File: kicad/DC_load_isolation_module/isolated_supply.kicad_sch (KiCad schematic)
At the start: 53 parts, among them Q10 AO3400A, Q11 AO3400A, Q12 MMBT5551L, Q14 MMBT5401, Q15 MMBT5551L, Q16 MMBT5551L, Q8 MMBT5551L, Q9 MMBT5401, U5 74HC14D653

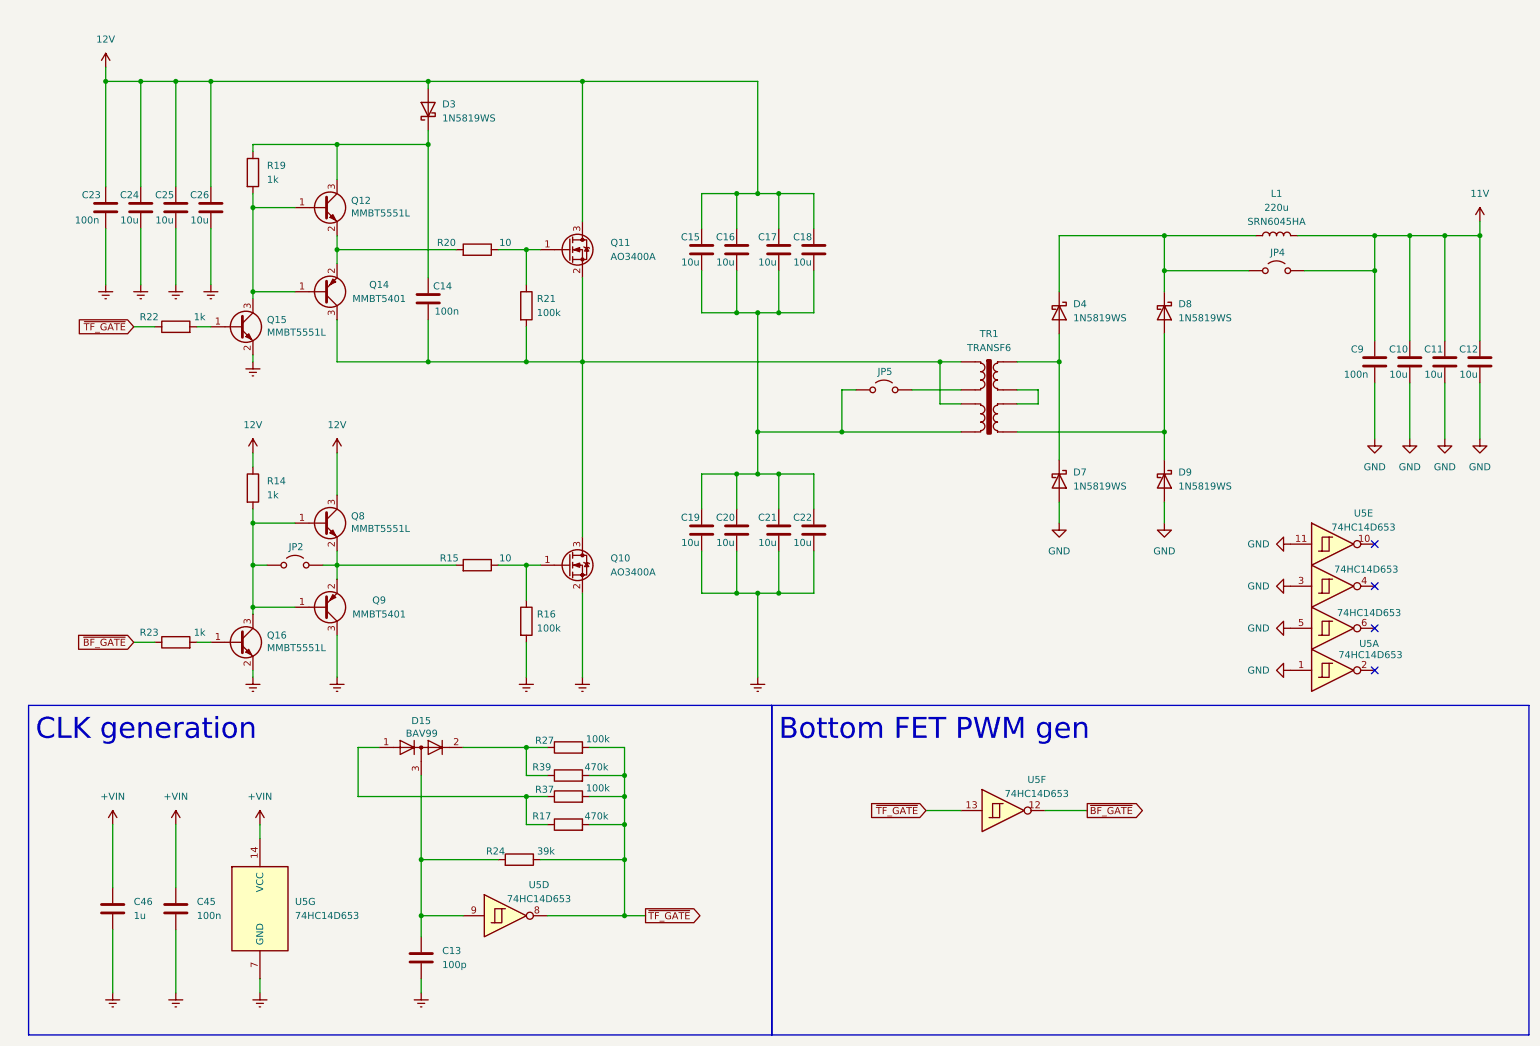
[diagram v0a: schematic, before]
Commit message: kk
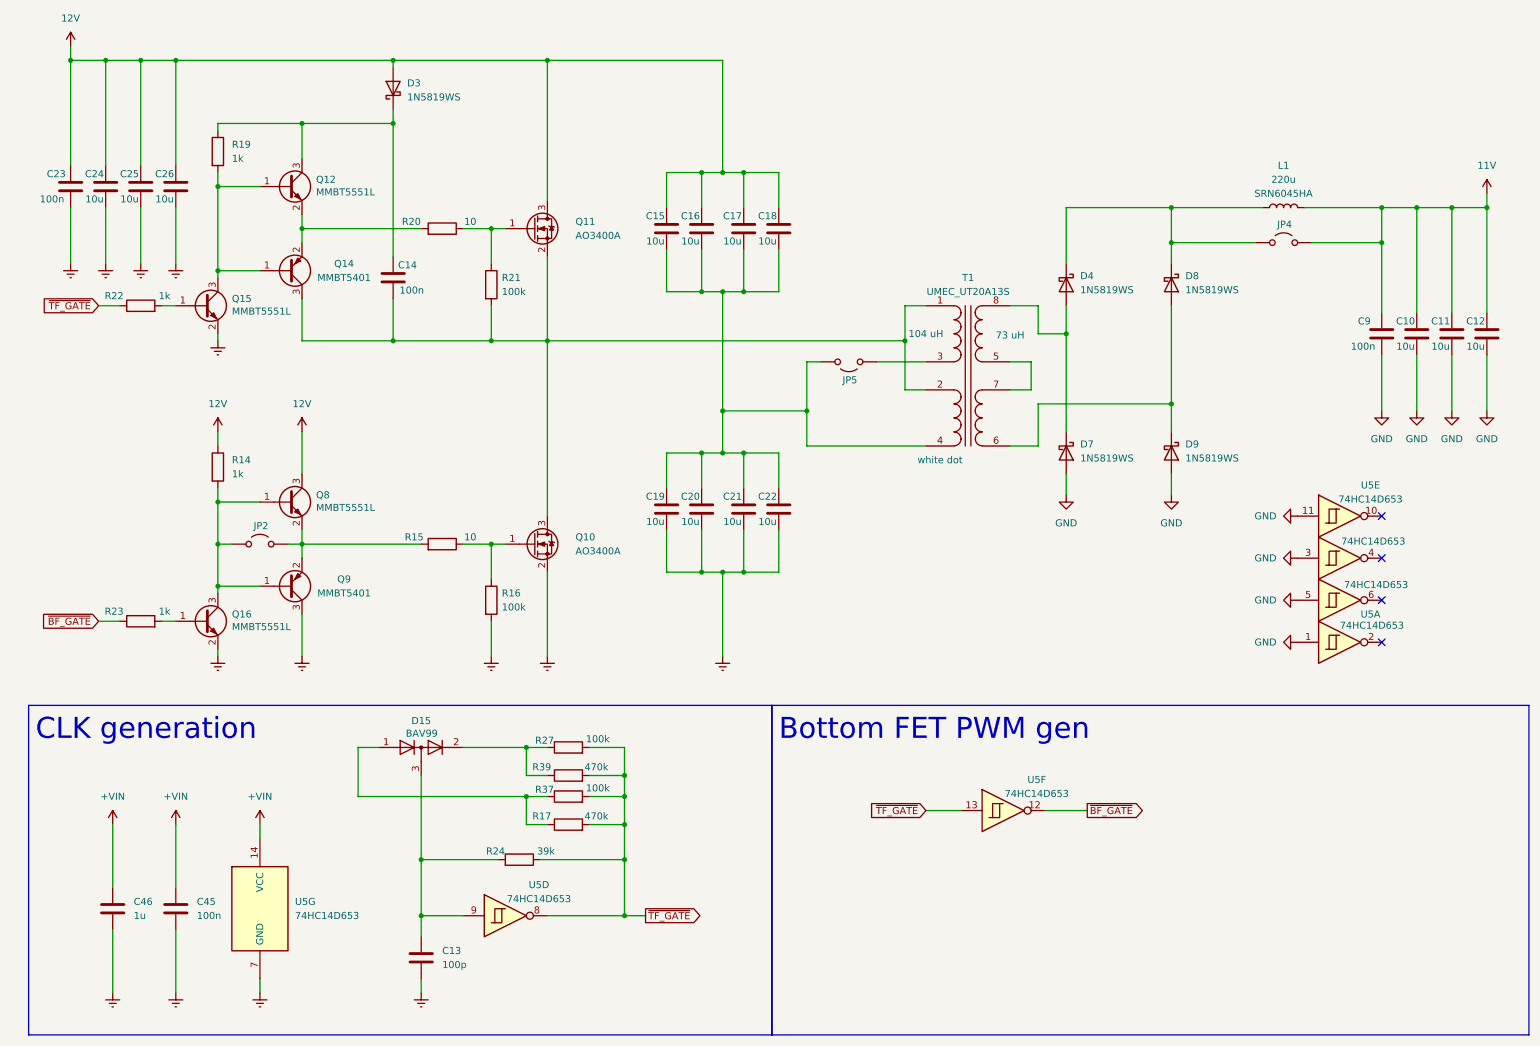
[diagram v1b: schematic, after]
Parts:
- removed TR1: TRANSF6, symbol Transformer:TRANSF6
- added T1: UMEC_UT20A13S, DC_load:UMEC_UT20A13S, symbol is:UMEC_UT20A13S
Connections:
- net at C14.2, Q10.3 (D), Q11.2 (S)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: now also T1.1 (AA), T1.2 (AA)
- net at C15.2, C16.2, C17.2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: now also T1.4 (AB)
- net at JP5.2 (B): now also T1.3 (AB)
- net at D8.2 (A), D9.1 (K): now also T1.6 (SA)
- net at D4.2 (A), D7.1 (K): now also T1.8 (SB)
- new net: T1.5 (SA), T1.7 (SB)
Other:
- moved on the sheet: C10, C11, C12, C14, C15, C16, C17, C18, C19, C20, C21, C22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
